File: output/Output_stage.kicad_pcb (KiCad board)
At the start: 2 copper layers, 62.9 x 27.9 mm, 16 parts, among them J1 Conn_01x03_Socket, J2 Control/LED, J3 Control/LED, Q1 BTA41, U1 MOC3041M

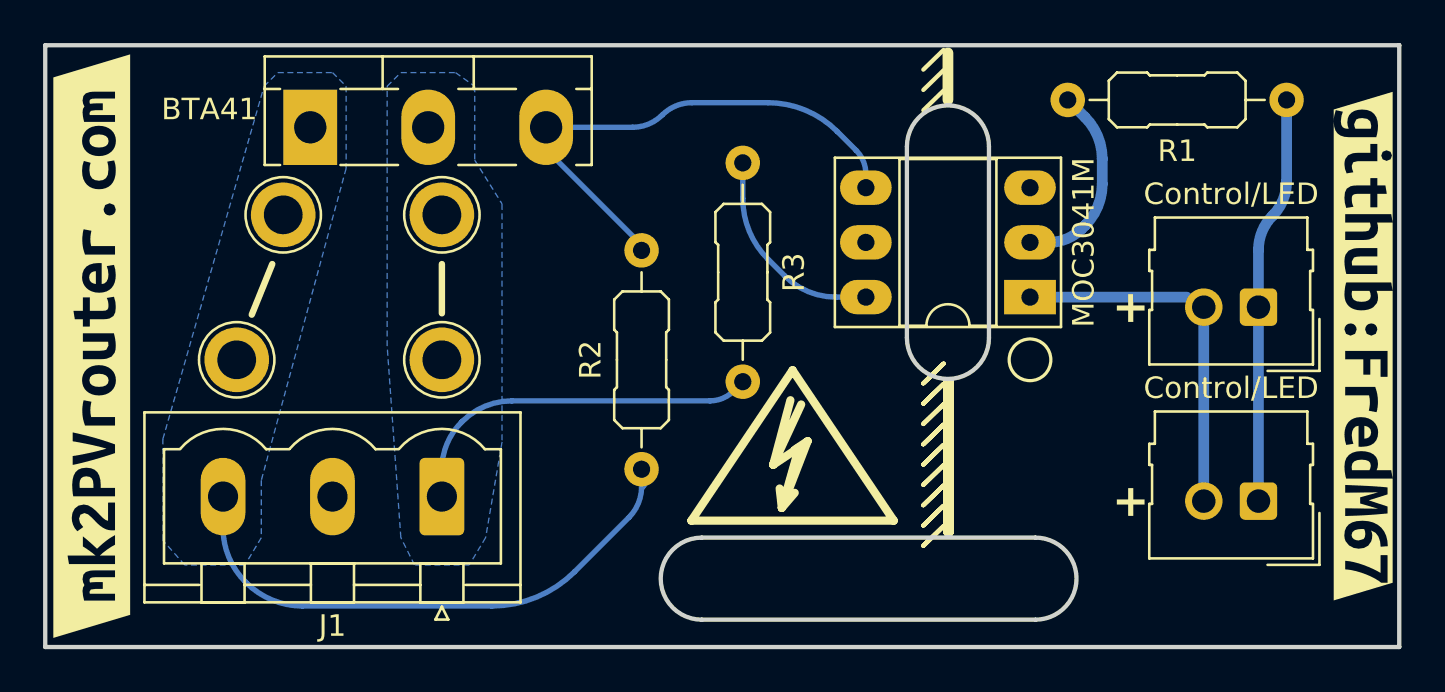
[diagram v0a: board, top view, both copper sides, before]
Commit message: Tiny tuning
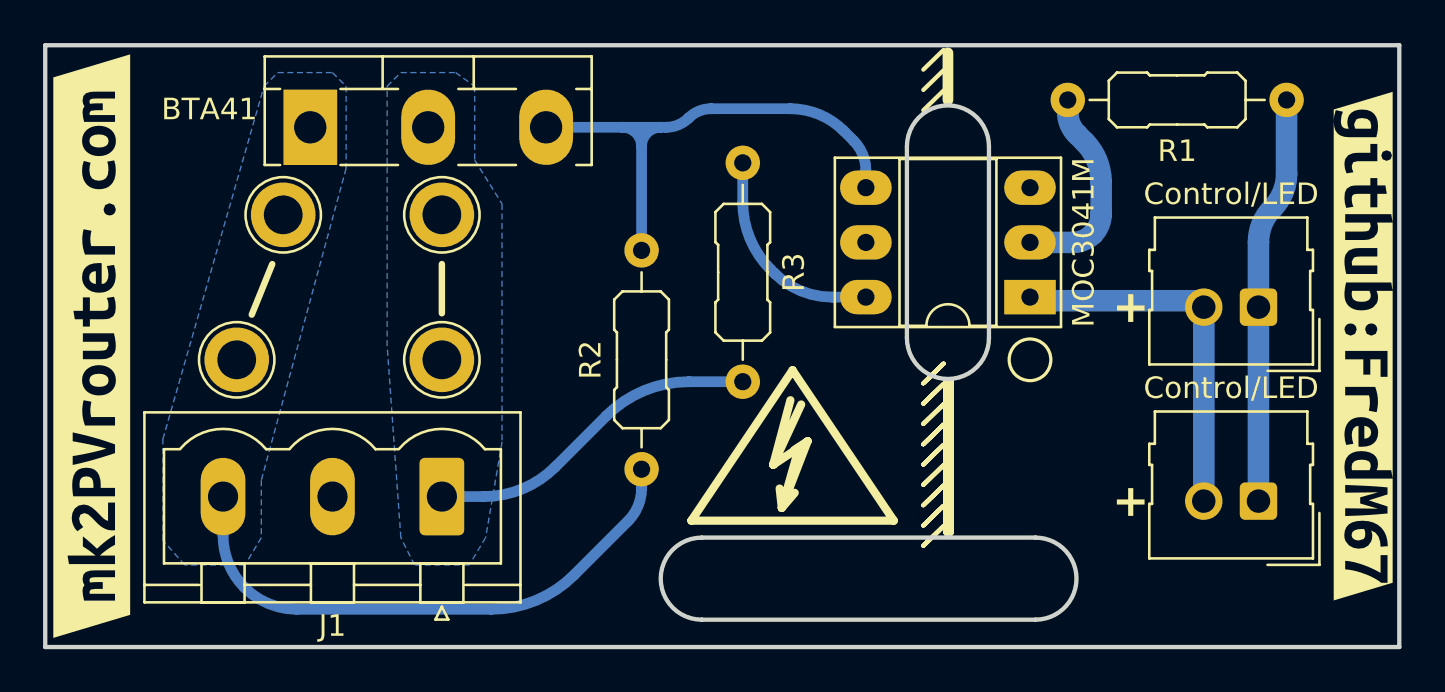
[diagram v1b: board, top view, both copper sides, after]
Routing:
- net LINE: track 17.3 -> 15.7 mm
- net Net-(J2-Pin_1): track 19.7 -> 19.0 mm
